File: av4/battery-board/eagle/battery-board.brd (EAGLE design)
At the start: 71.2 x 35.3 mm, 59 parts, among them J100 ROCKETNET-BATTERY-14, J101 87758-0216, J102 87758-0216, Q100 Si2343DS-T1, Q101 SI4435DDY, Q102 SI4435DDY, Q103 SI1023X, Q104 SI1023X, U100 BQ3060PW

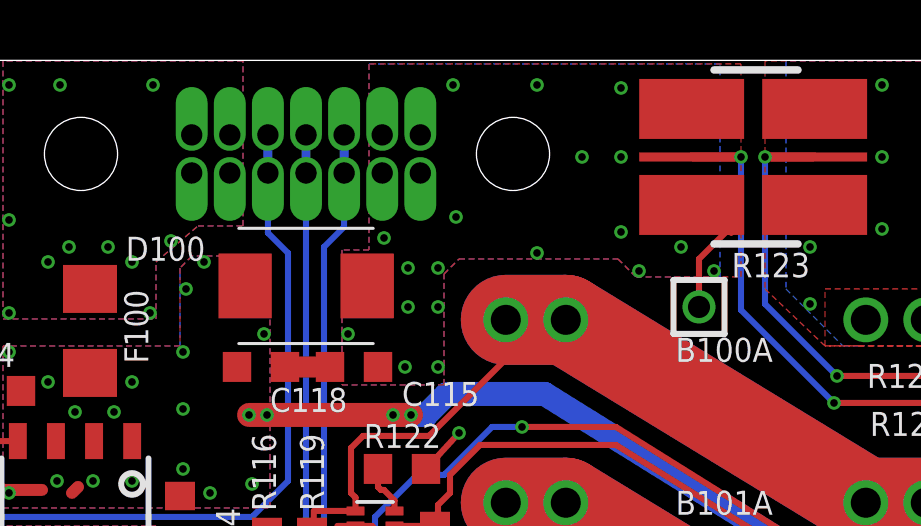
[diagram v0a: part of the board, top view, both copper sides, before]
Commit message: Generated BOM and made a Digi-Key order. Found an ERC error that popped up, double checked part values in writeup.
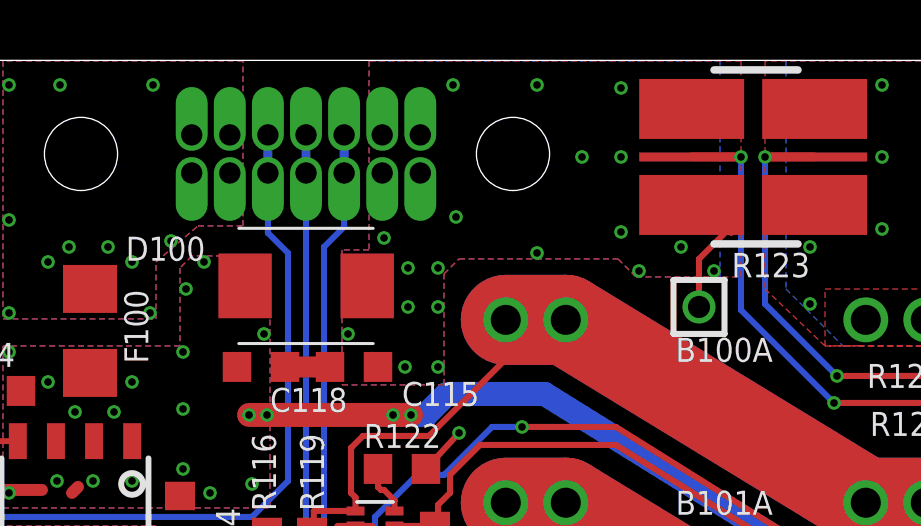
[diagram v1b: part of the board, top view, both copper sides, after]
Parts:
- Q101, Q102: value SI4435DDY -> SI4413ADY-T1-E3
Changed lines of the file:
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@@
 <layers>
 <layer number="1" name="Top" color="4" fill="1" visible="yes" active="yes"/>
-<layer number="2" name="Route2" color="15" fill="1" visible="yes" active="yes"/>
-<layer number="3" name="Route3" color="11" fill="1" visible="yes" active="yes"/>
+<layer number="2" name="Route2" color="15" fill="1" visible="no" active="yes"/>
+<layer number="3" name="Route3" color="11" fill="1" visible="no" active="yes"/>
 <layer number="4" name="Route4" color="1" fill="4" visible="no" active="no"/>
 <layer number="5" name="Route5" color="4" fill="4" visible="no" active="no"/>
@@
 <layer number="27" name="tValues" color="7" fill="1" visible="no" active="yes"/>
 <layer number="28" name="bValues" color="7" fill="1" visible="no" active="yes"/>
-<layer number="29" name="tStop" color="7" fill="3" visible="yes" active="yes"/>
+<layer number="29" name="tStop" color="7" fill="3" visible="no" active="yes"/>
 <layer number="30" name="bStop" color="7" fill="6" visible="no" active="yes"/>
 <layer number="31" name="tCream" color="7" fill="4" visible="no" active="yes"/>
@@
 <element name="TP107" library="Tova" package="2MM-TEST-POINT" value="TEST-POINT" x="62.6" y="16.5" smashed="yes"/>
 <element name="TP108" library="Tova" package="2MM-TEST-POINT" value="TEST-POINT" x="62.6" y="14.5"/>
-<element name="Q101" library="si4435ddy" package="SO-8" value="SI4435DDY" x="14.2" y="12" smashed="yes">
+<element name="Q101" library="si4435ddy" package="SO-8" value="SI4413ADY-T1-E3" x="14.2" y="12" smashed="yes">
 <attribute name="NAME" x="11.5" y="10.9" size="0.8128" layer="25" font="vector" ratio="20" rot="R90"/>
 </element>
-<element name="Q102" library="si4435ddy" package="SO-8" value="SI4435DDY" x="14.2" y="20.1" smashed="yes" rot="R180">
+<element name="Q102" library="si4435ddy" package="SO-8" value="SI4413ADY-T1-E3" x="14.2" y="20.1" smashed="yes" rot="R180">
 <attribute name="NAME" x="10.6" y="21.6" size="0.8128" layer="25" font="vector" ratio="20" rot="R270"/>
 </element>
@@
 <via x="45.798" y="12.39" extent="1-16" drill="0.254"/>
 <via x="45.798" y="14.39" extent="1-16" drill="0.254"/>
-<wire x1="22.3" y1="23.1" x2="22.3" y2="22.9" width="0.2032" layer="2"/>
 <polygon width="0.2" layer="3" isolate="0.4" rank="6">
 <vertex x="71.2" y="35.3"/>
@@
 <wire x1="25.9" y1="21.7" x2="27" y2="22.9" width="0.2032" layer="1"/>
 <via x="27" y="22.9" extent="1-16" drill="0.254"/>
-<wire x1="27" y1="22.9" x2="27.1" y2="22.9" width="0.2032" layer="2"/>
 <via x="42.7" y="32.1" extent="1-16" drill="0.254"/>
 <via x="45" y="32.1" extent="1-16" drill="0.254"/>
@@
 <contactref element="C115" pad="2"/>
 <polygon width="0.2" layer="1" isolate="0.2" thermals="no" rank="3">
-<vertex x="24" y="35.2"/>
+<vertex x="24" y="35.3"/>
 <vertex x="24" y="29"/>
 <vertex x="23.1" y="29"/>
@@
 <vertex x="32.9" y="28.1"/>
 <vertex x="36.4" y="28.1"/>
-<vertex x="36.4" y="35.2"/>
+<vertex x="36.4" y="35.3"/>
 </polygon>
 <contactref element="J100" pad="B-@11"/>
@@
 <vertex x="23.1" y="29"/>
 <vertex x="23.1" y="24.5"/>
-<vertex x="26.4" y="24.5"/>
-<vertex x="26.4" y="27.2"/>
-<vertex x="27.3" y="28.1"/>
-<vertex x="36" y="28.1"/>
-<vertex x="36" y="35.3"/>
+<vertex x="26.5" y="24.5"/>
+<vertex x="26.5" y="28.2"/>
+<vertex x="27" y="28.7"/>
+<vertex x="32.3" y="28.7"/>
+<vertex x="32.9" y="28.1"/>
+<vertex x="35.7" y="28.1"/>
+<vertex x="35.7" y="35.3"/>
 </polygon>
 <polygon width="0.2" layer="3" isolate="0.4" thermals="no" rank="2">
 <vertex x="24" y="35.3"/>
-<vertex x="24" y="29"/>
-<vertex x="23.1" y="29"/>
-<vertex x="23.1" y="24.5"/>
-<vertex x="26.4" y="24.5"/>
-<vertex x="26.4" y="27.2"/>
-<vertex x="27.3" y="28.1"/>
-<vertex x="36" y="28.1"/>
-<vertex x="36" y="35.3"/>
-</polygon>
-<polygon width="0.2" layer="16" isolate="0.2" thermals="no" rank="3">
-<vertex x="24" y="35.2"/>
 <vertex x="24" y="29"/>
 <vertex x="23.1" y="29"/>
@@
 <vertex x="32.9" y="28.1"/>
 <vertex x="35.7" y="28.1"/>
-<vertex x="35.7" y="35.2"/>
+<vertex x="35.7" y="35.3"/>
+</polygon>
+<polygon width="0.2" layer="16" isolate="0.2" thermals="no" rank="3">
+<vertex x="24" y="35.3"/>
+<vertex x="24" y="29"/>
+<vertex x="23.1" y="29"/>
+<vertex x="23.1" y="24.5"/>
+<vertex x="26.5" y="24.5"/>
+<vertex x="26.5" y="28.2"/>
+<vertex x="27" y="28.7"/>
+<vertex x="32.3" y="28.7"/>
+<vertex x="32.9" y="28.1"/>
+<vertex x="35.7" y="28.1"/>
+<vertex x="35.7" y="35.3"/>
 </polygon>
 <via x="32.4" y="34.4" extent="1-16" drill="0.254"/>
@@
 <vertex x="20.7" y="20.4"/>
 <vertex x="20.7" y="28.8"/>
-<vertex x="17.7" y="28.8"/>
+<vertex x="18.1" y="28.8"/>
+<vertex x="17.7" y="28.4"/>
 <vertex x="17.7" y="25.8"/>
 </polygon>
@@
 <vertex x="20.7" y="20.4"/>
 <vertex x="20.7" y="28.8"/>
-<vertex x="17.7" y="28.8"/>
+<vertex x="18.1" y="28.8"/>
+<vertex x="17.7" y="28.4"/>
 <vertex x="17.7" y="25.8"/>
 </polygon>
@@
 <vertex x="18.1" y="28.8"/>
 <vertex x="17.7" y="28.4"/>
-<vertex x="17.7" y="28.2"/>
 <vertex x="17.7" y="25.8"/>
 </polygon>
@@
 <vertex x="11.8" y="26.7"/>
 <vertex x="16.9" y="26.7"/>
-<vertex x="16.9" y="28.5"/>
-<vertex x="18.4" y="29.8"/>
+<vertex x="16.9" y="28.6"/>
+<vertex x="18.3" y="29.8"/>
 </polygon>
 <polygon width="0.2" layer="3" isolate="0.4" thermals="no" rank="2">
@@
 <vertex x="11.8" y="26.7"/>
 <vertex x="16.9" y="26.7"/>
-<vertex x="16.9" y="28.5"/>
-<vertex x="18.4" y="29.8"/>
+<vertex x="16.9" y="28.6"/>
+<vertex x="18.3" y="29.8"/>
 </polygon>
 <via x="17.4" y="29.3" extent="1-16" drill="0.254"/>
